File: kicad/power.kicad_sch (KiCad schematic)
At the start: 32 parts, among them IC1 RT6254BHGJ6F, IC3 RT6254BHGJ6F, U3 TLV75733PDBVR

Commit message: finish first pcb revision
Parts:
- C1, C4: footprint (none) -> 25TQC100MD3:16TDC150MYF
- C26, C3: footprint (none) -> 10TPE220ML:16TDC150MYF
- C30, C32: footprint (none) -> Capacitor_SMD:C_0201_0603Metric
- FB1: footprint (none) -> BLM21PG300SN1D:BEADC2012X105N
- IC1, IC3: footprint (none) -> RT6254BHGJ6F:SOT95P280X100-6N
- L1, L3: footprint (none) -> ETQP3M4R7KVN:ETQP3M1R0KVN
- U3: footprint (none) -> TLV75733PDBVR:DBV0005A_N
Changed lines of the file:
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@@
 			)
 		)
-		(property "Footprint" ""
+		(property "Footprint" "RT6254BHGJ6F:SOT95P280X100-6N"
 			(at 120.65 205.41 0)
 			(effects
@@
 			)
 		)
-		(property "Footprint" ""
+		(property "Footprint" "RT6254BHGJ6F:SOT95P280X100-6N"
 			(at 120.65 144.45 0)
 			(effects
@@
 		)
 		(instances
-			(project ""
+			(project "hammerhead_sensor_module"
 				(path "/5313a223-fa0e-4103-9806-d293f3d5507a/8293f066-7499-4d50-94d4-999fc085e2c1"
 					(reference "IC1")
@@
 			)
 		)
-		(property "Footprint" ""
+		(property "Footprint" "25TQC100MD3:16TDC150MYF"
 			(at -46.66 58.42 0)
 			(effects
@@
 		)
 		(instances
-			(project ""
+			(project "hammerhead_sensor_module"
 				(path "/5313a223-fa0e-4103-9806-d293f3d5507a/8293f066-7499-4d50-94d4-999fc085e2c1"
 					(reference "C1")
@@
 			)
 		)
-		(property "Footprint" ""
+		(property "Footprint" "BLM21PG300SN1D:BEADC2012X105N"
 			(at 318.44 93.98 0)
 			(effects
@@
 		)
 		(instances
-			(project ""
+			(project "hammerhead_sensor_module"
 				(path "/5313a223-fa0e-4103-9806-d293f3d5507a/8293f066-7499-4d50-94d4-999fc085e2c1"
 					(reference "FB1")
@@
 			)
 		)
-		(property "Footprint" ""
+		(property "Footprint" "ETQP3M4R7KVN:ETQP3M1R0KVN"
 			(at 160.02 206.68 0)
 			(effects
@@
 			)
 		)
-		(property "Footprint" ""
+		(property "Footprint" "ETQP3M4R7KVN:ETQP3M1R0KVN"
 			(at 160.02 145.72 0)
 			(effects
@@
 		)
 		(instances
-			(project ""
+			(project "hammerhead_sensor_module"
 				(path "/5313a223-fa0e-4103-9806-d293f3d5507a/8293f066-7499-4d50-94d4-999fc085e2c1"
 					(reference "L1")
@@
 			)
 		)
-		(property "Footprint" ""
+		(property "Footprint" "TLV75733PDBVR:DBV0005A_N"
 			(at 111.76 170.18 0)
 			(effects
@@
 		)
 		(instances
-			(project ""
+			(project "hammerhead_sensor_module"
 				(path "/5313a223-fa0e-4103-9806-d293f3d5507a/8293f066-7499-4d50-94d4-999fc085e2c1"
 					(reference "U3")
@@
 			)
 		)
-		(property "Footprint" ""
+		(property "Footprint" "Capacitor_SMD:C_0201_0603Metric"
 			(at 88.5952 170.18 0)
 			(effects
@@
 		)
 		(instances
-			(project ""
+			(project "hammerhead_sensor_module"
 				(path "/5313a223-fa0e-4103-9806-d293f3d5507a/8293f066-7499-4d50-94d4-999fc085e2c1"
 					(reference "C30")
@@
 			)
 		)
-		(property "Footprint" ""
+		(property "Footprint" "25TQC100MD3:16TDC150MYF"
 			(at -46.66 119.38 0)
 			(effects
@@
 			)
 		)
-		(property "Footprint" ""
+		(property "Footprint" "Capacitor_SMD:C_0201_0603Metric"
 			(at 129.2352 170.18 0)
 			(effects
@@
 			)
 		)
-		(property "Footprint" ""
+		(property "Footprint" "10TPE220ML:16TDC150MYF"
 			(at 127.33 58.42 0)
 			(effects
@@
 		)
 		(instances
-			(project ""
+			(project "hammerhead_sensor_module"
 				(path "/5313a223-fa0e-4103-9806-d293f3d5507a/8293f066-7499-4d50-94d4-999fc085e2c1"
 					(reference "C3")
@@
 			)
 		)
-		(property "Footprint" ""
+		(property "Footprint" "10TPE220ML:16TDC150MYF"
 			(at 142.57 119.38 0)
 			(effects

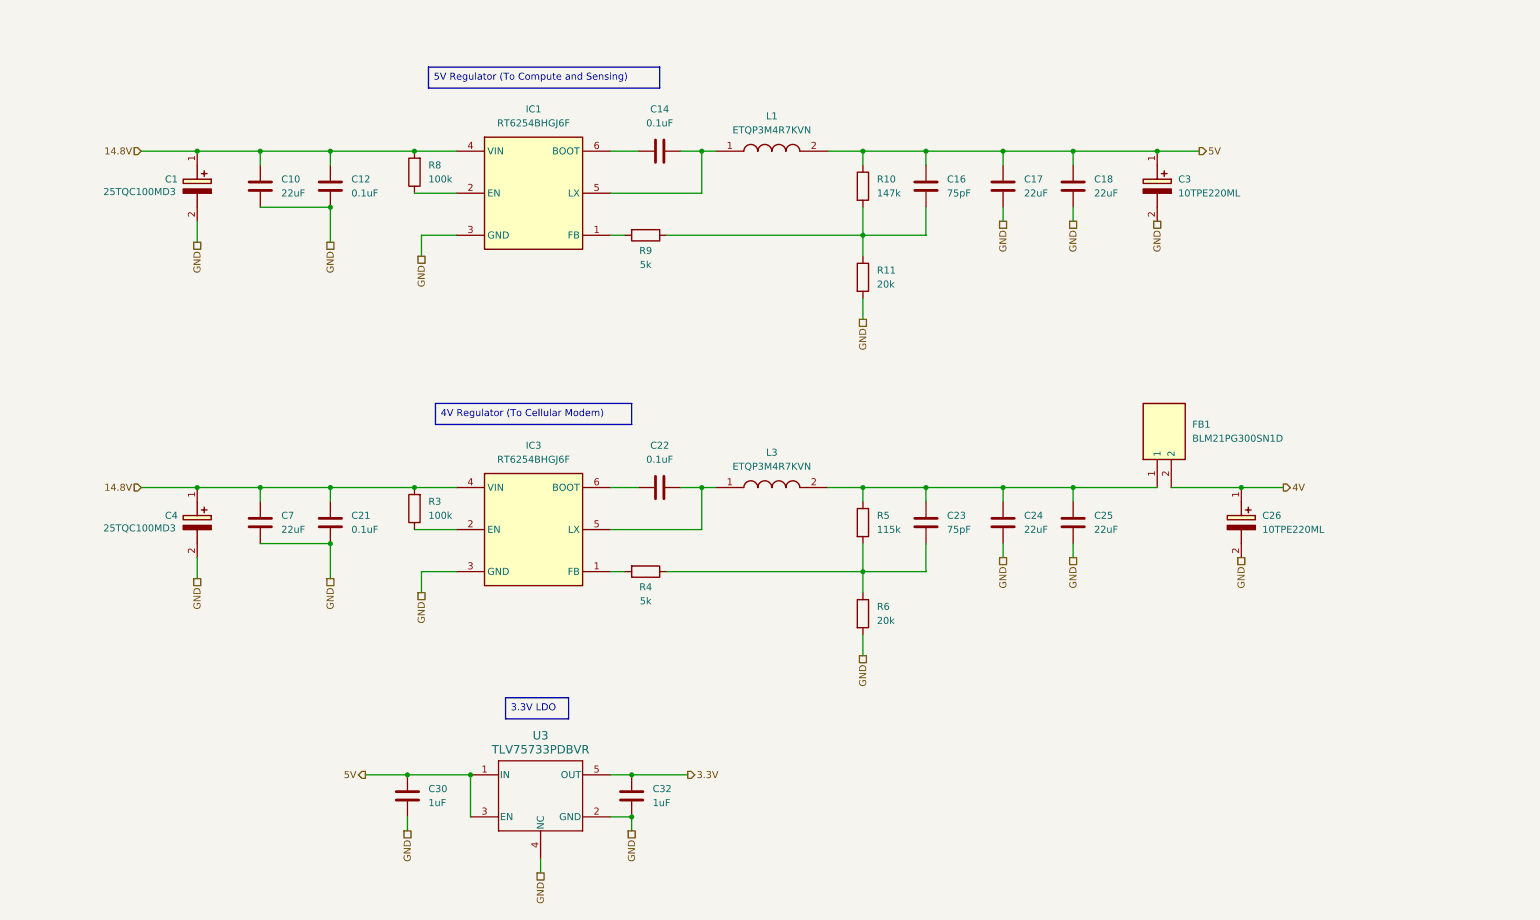
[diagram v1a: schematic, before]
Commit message: add docs and cleanup
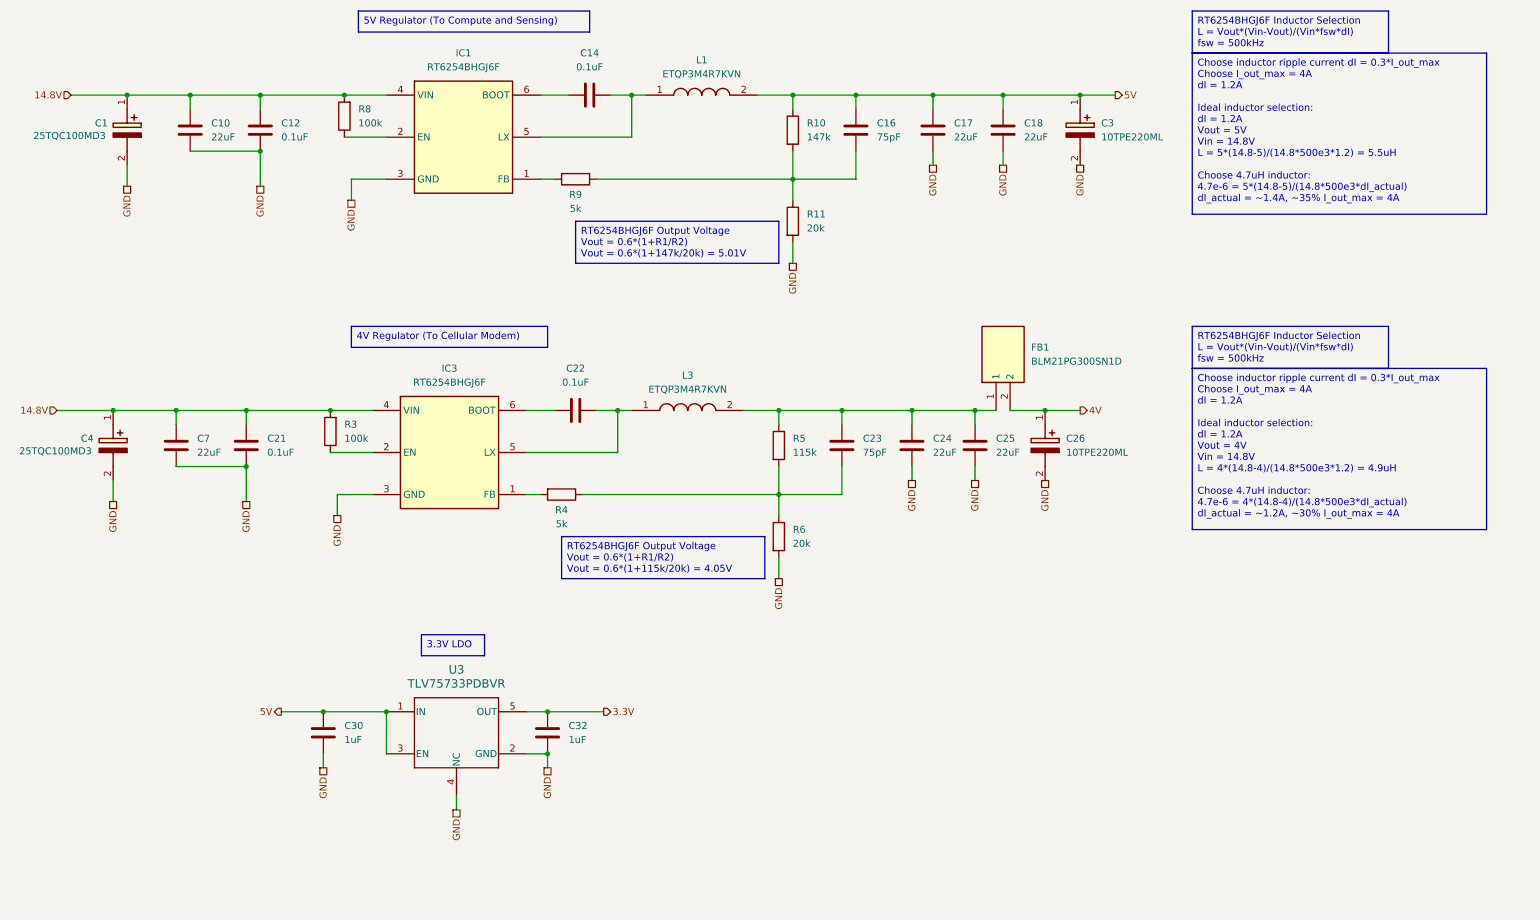
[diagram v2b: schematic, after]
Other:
- moved on the sheet: C1, C10, C12, C14, C16, C17, C18, C21, C22, C23, C24, C25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

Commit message: generate manufacturing files, final checks, cleanup
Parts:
- R10, R5: footprint Resistor_SMD:R_0201_0603Metric -> Resistor_SMD:R_0402_1005Metric
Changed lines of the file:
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@@
 			)
 		)
-		(property "Footprint" "Resistor_SMD:R_0201_0603Metric"
+		(property "Footprint" "Resistor_SMD:R_0402_1005Metric"
 			(at 153.162 102.87 90)
 			(effects
@@
 			)
 		)
-		(property "Footprint" "Resistor_SMD:R_0201_0603Metric"
+		(property "Footprint" "Resistor_SMD:R_0402_1005Metric"
 			(at 155.702 45.72 90)
 			(effects
